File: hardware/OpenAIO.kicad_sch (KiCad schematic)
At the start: 8 parts, among them J1 OpenDrone-Core, U24 AIO_outline, U25 INA186A3IDCKR

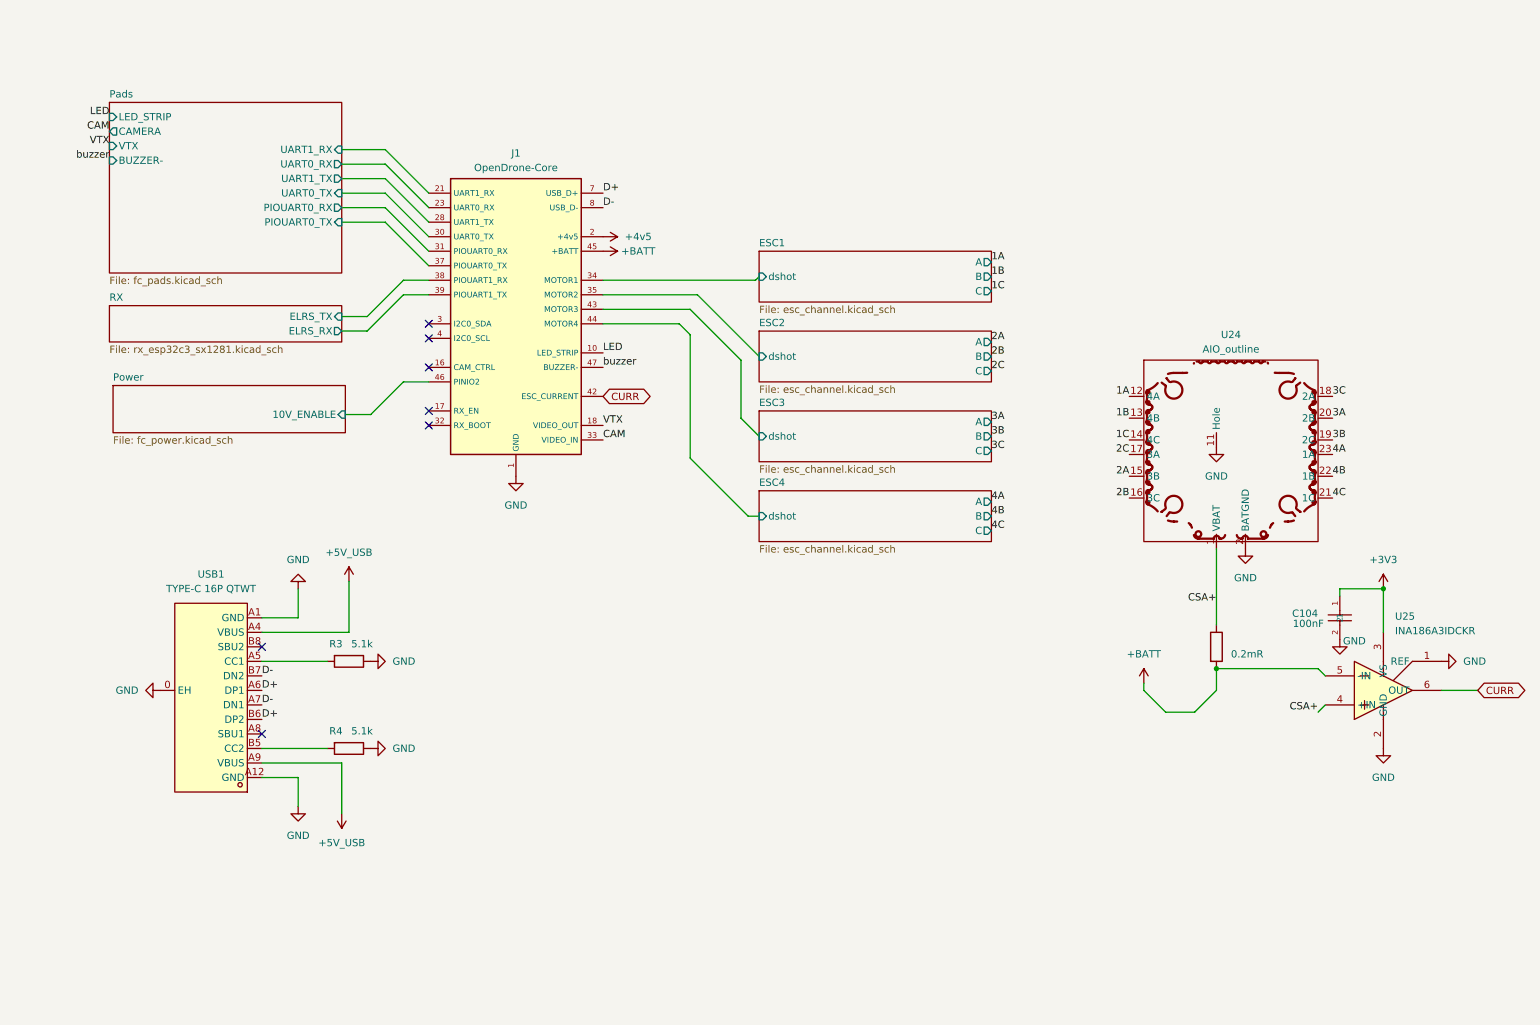
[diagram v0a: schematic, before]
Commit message: chore: consolidate OpenAIO design assets and guidance
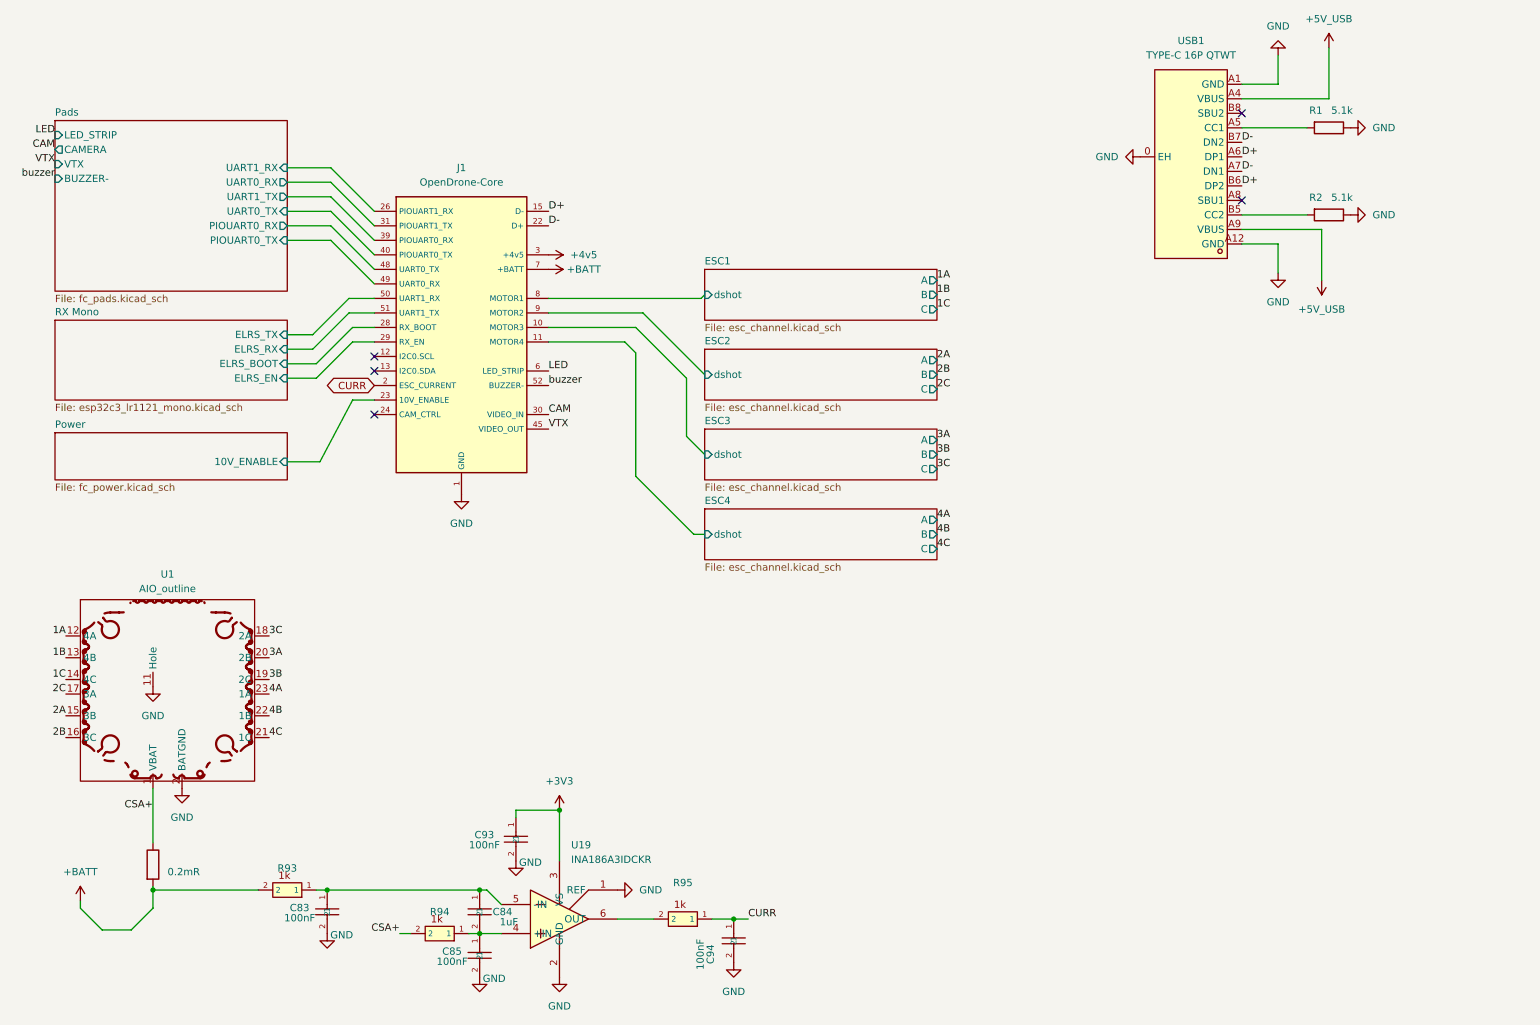
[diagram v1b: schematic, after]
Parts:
- removed C104: 100nF, Capacitor_SMD:C_0201_0603Metric, symbol ESCLibrary:GRM033R61C104KE84D
- removed U25: INA186A3IDCKR, 4in1ESC:SOT-363_SC-70-6, symbol components:INA186A3IDCKR
- added C83, C85: 100nF, Capacitor_SMD:C_0402_WIDE, symbol ESCLibrary:GRM033R61C104KE84D
- added C84: 1uF, Capacitor_SMD:C_0402_1005Metric, symbol ESCLibrary:GRM033R61C104KE84D
- added C93, C94: 100nF, Capacitor_SMD:C_0201_0603Metric, symbol ESCLibrary:GRM033R61C104KE84D
- added R93, R94: 1k, Capacitor_SMD:C_0201_0603Metric, symbol components:0201_1kR
- added R95: 1k, 4in1ESC:R_0201_0603Metric, symbol ESCLibrary:0201_1kR
- added U19: INA186A3IDCKR, 4in1ESC:SOT-363_SC-70-6, symbol components:INA186A3IDCKR
- Rsense2: KiLib_Generator SMD_2terminal_chip_molded -> (none); Manufacturer (none) -> Yezhan
- renumbered R3 to R1, R4 to R2, U24 to U1
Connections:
- net RX/ELRS_RX is gone; now on net Pads/UART1_TX: J1.39 (PIOUART0_RX)
- net RX/ELRS_TX is gone; now on net GND: J1.38 (GND)
- net +3V3: now also C93.1, U19.3 (VS)
- net +4v5: now also J1.3 (+4v5); no longer J1.2 (+4v5)
- net +BATT: now also J1.7 (+BATT), R93.2; no longer J1.45 (+BATT)
- net CAM: now also J1.30 (VIDEO_IN); no longer J1.33 (VIDEO_IN)
- net CSA+: now also R94.2
- net CURR: now also J1.2 (ESC_CURRENT), C94.1, R95.1; no longer J1.42 (ESC_CURRENT)
- net D+: now also J1.15 (D-); no longer J1.7 (USB_D+)
- net D-: now also J1.22 (D+); no longer J1.8 (USB_D-)
- net ESC1/dshot: now also J1.8 (MOTOR1); no longer J1.34 (MOTOR1)
- net ESC2/dshot: now also J1.9 (MOTOR2); no longer J1.35 (MOTOR2)
- net ESC3/dshot: now also J1.10 (MOTOR3); no longer J1.43 (MOTOR3)
- net ESC4/dshot: now also J1.11 (MOTOR4); no longer J1.44 (MOTOR4)
- net GND: now also J1.16 (GND), J1.17 (GND), J1.18 (GND), J1.21 (GND), J1.32 (GND), J1.33 (GND), J1.34 (GND), J1.35 (GND), J1.37 (GND), J1.4 (GND), J1.42 (GND), J1.43 (GND), J1.44 (GND), J1.46 (GND), J1.47 (GND), C83.2, C85.2, C93.2, C94.2, U19.1 (REF), U19.2 (GND); no longer J1.11 (GND), J1.12 (GND), J1.13 (GND), J1.15 (GND), J1.22 (GND), J1.24 (GND), J1.26 (GND), J1.29 (GND), J1.40 (GND), J1.48 (GND), J1.49 (GND), J1.50 (GND), J1.51 (GND), J1.52 (GND), J1.53 (GND), J1.54 (GND), J1.6 (GND), J1.9 (GND)
- net LED: now also J1.6 (LED_STRIP); no longer J1.10 (LED_STRIP)
- net Pads/PIOUART0_RX: now also J1.48 (UART0_TX); no longer J1.31 (PIOUART0_RX)
- net Pads/PIOUART0_TX: now also J1.49 (UART0_RX); no longer J1.37 (PIOUART0_TX)
- net Pads/UART0_RX: now also J1.31 (PIOUART1_TX); no longer J1.23 (UART0_RX)
- net Pads/UART0_TX: now also J1.40 (PIOUART0_TX); no longer J1.30 (UART0_TX)
- net Pads/UART1_RX: now also J1.26 (PIOUART1_RX); no longer J1.21 (UART1_RX)
- net Pads/UART1_TX: no longer J1.28 (UART1_TX)
- net Power/10V_ENABLE: now also J1.23 (10V_ENABLE); no longer J1.46 (PINIO2)
- net VTX: now also J1.45 (VIDEO_OUT); no longer J1.18 (VIDEO_OUT)
- net buzzer: now also J1.52 (BUZZER-); no longer J1.47 (BUZZER-)
- new net: C83.1, C84.1, R93.1, U19.5 (-IN)
- new net: C84.2, C85.1, R94.1, U19.4 (+IN)
- new net: R95.2, U19.6 (OUT)
- new net RX Mono/ELRS_BOOT: J1.28 (RX_BOOT)
- new net RX Mono/ELRS_EN: J1.29 (RX_EN)
- new net RX Mono/ELRS_RX: J1.51 (UART1_TX)
- new net RX Mono/ELRS_TX: J1.50 (UART1_RX)
- no-connect marks 7 -> 5
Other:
- removed sheet RX
- added sheet RX Mono (esp32c3_lr1121_mono.kicad_sch)
- moved on the sheet: R1, R2, U1, USB1
